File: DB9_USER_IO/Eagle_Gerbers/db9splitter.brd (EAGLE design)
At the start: 62.5 x 19.8 mm, 19 parts, among them IC1 74LVC1G04DBV

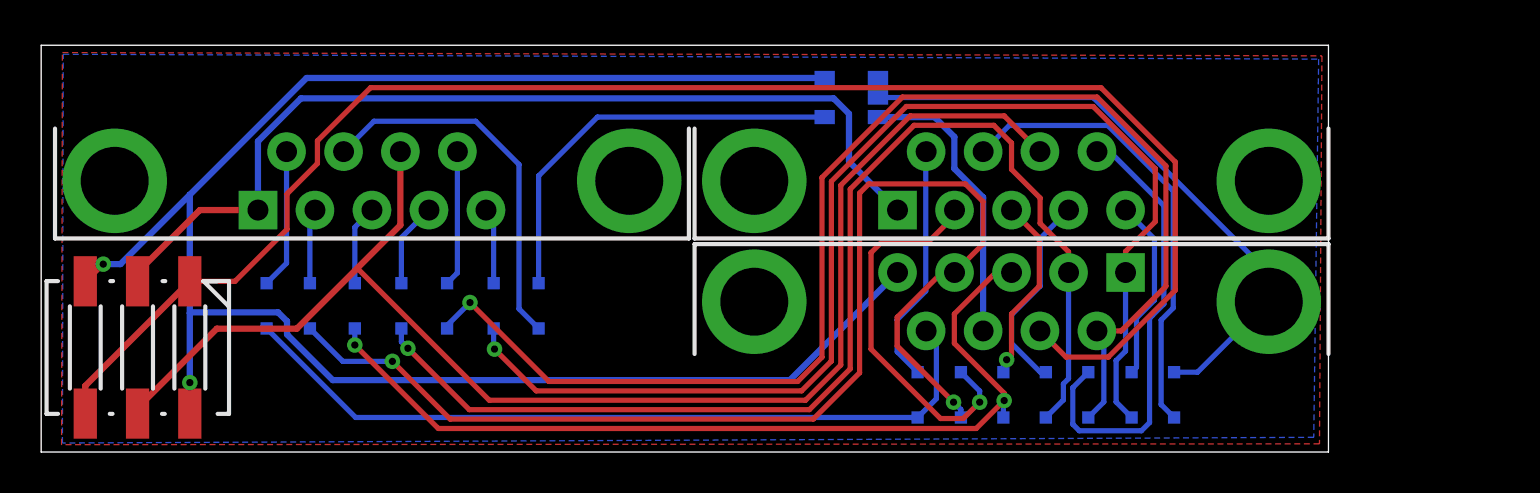
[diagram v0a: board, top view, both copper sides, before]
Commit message: updated db9splitter
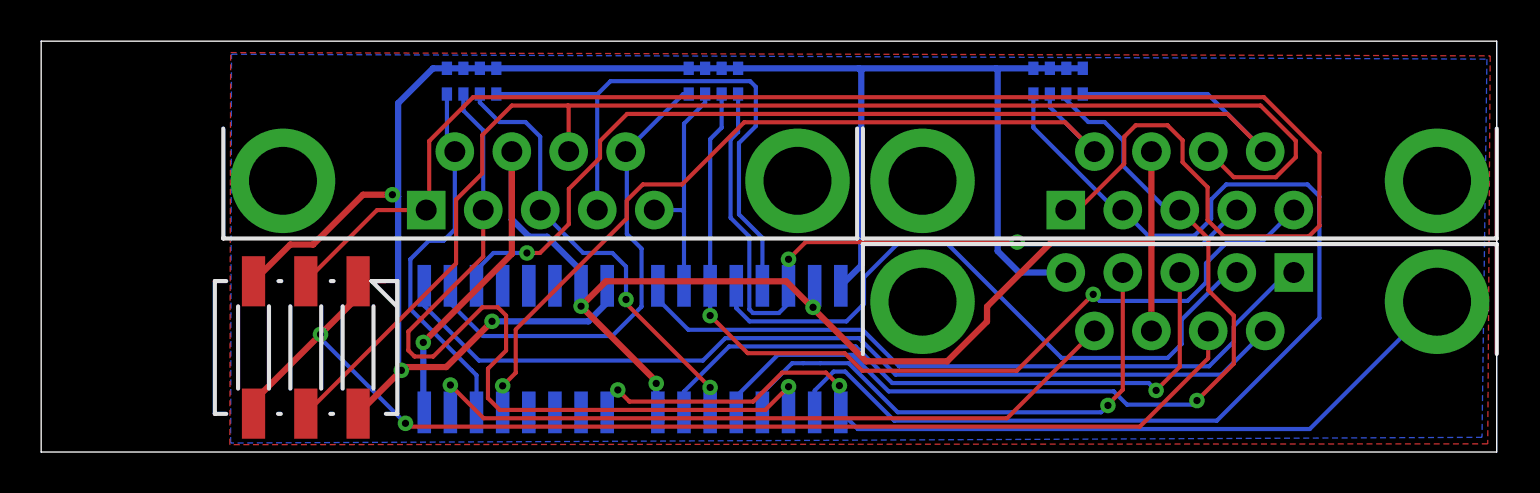
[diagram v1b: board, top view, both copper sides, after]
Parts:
- removed D1, D10, D11, D12, D13, D14, D2, D3, D4, D5, D6, D7, D8, D9: (no value), diode:SOD323-R
- removed IC1: 74LVC1G04DBV, 74xx-little-de:SOT23-5
- added IC2, IC3: 74HC157D, 74xx-eu:SO16
- added RN2, RN3, RN5: 10K, resistor-dil:0603-ARC
- moved J1 8.18 mm to (55.3, 13.2)
- moved J2 8.18 mm to (55.3, 7.30)
- moved J3 8.18 mm to (24.2, 13.2)
- moved S1 8.18 mm to (12.9, 5.08)
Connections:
- removed net /SELECT: D10.C, IC1.4
- removed net N$1: D13.C, J1.1
- removed net N$11: D6.C, J1.9
- removed net N$12: D5.C, J1.6
- removed net N$13: D12.C, J3.9
- removed net N$14: D11.C, J3.6
- removed net N$15: D4.A, J1.8
- removed net N$2: D14.C, J3.1
- removed net N$3: D2.C, J1.3
- removed net N$4: D8.C, J3.3
- removed net N$5: D1.C, J1.2
- removed net N$6: D3.C, J1.4
- removed net N$7: D7.C, J3.2
- removed net N$8: D9.C, J3.4
- removed net N$9: D10.A, J3.8
- new net 1PDOWN: IC2.14, J1.2, RN2.1
- new net 1PFIRE1: IC3.11, J1.6, RN5.1
- new net 1PFIRE2: IC3.5, J1.9, RN5.3
- new net 1PLEFT: IC2.5, J1.3, RN5.2
- new net 1PRIGHT: IC2.2, J1.4, RN5.4
- new net 1PUP: IC2.11, J1.1, RN2.2
- new net 2PDOWN: IC2.13, J3.2, RN3.1
- new net 2PFIRE1: IC3.10, J3.6, RN2.4
- new net 2PFIRE2: IC3.6, J3.9, RN3.4
- new net 2PLEFT: IC2.6, J3.3, RN3.2
- new net 2PRIGHT: IC2.3, J3.4, RN3.3
- new net 2PUP: IC2.10, J3.1, RN2.3
- net DOWN: now also IC2.12; no longer D1.A, D7.A
- net FIRE1: now also IC3.9; no longer D11.A, D5.A
- net FIRE2: now also IC3.7; no longer D12.A, D6.A
- net GND: now also IC2.15, IC2.8, IC3.15, IC3.8, J1.8, J3.8; no longer IC1.3
- net LEFT: now also IC2.7; no longer D2.A, D8.A
- net RIGHT: now also IC2.4; no longer D3.A, D9.A
- net SELECT: now also IC2.1, IC3.1; no longer D4.C, IC1.2
- net UP: now also IC2.9; no longer D13.A, D14.A
- net VCC: now also IC2.16, IC3.16, RN2.5, RN2.6, RN2.7, RN2.8, RN3.5, RN3.6, RN3.7, RN3.8, RN5.5, RN5.6, RN5.7, RN5.8; no longer IC1.5
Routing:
- net GND: track 14.1 -> 73.1 mm, vias 0 -> 4
- net 1PFIRE1: track 0.00 -> 54.5 mm, vias 0 -> 1
- net 1PRIGHT: track 0.00 -> 54.5 mm
- net 1PLEFT: track 0.00 -> 44.9 mm, vias 0 -> 1
- net 1PUP: track 0.00 -> 44.5 mm, vias 0 -> 2
- net 1PFIRE2: track 0.00 -> 41.4 mm, vias 0 -> 1
- net 2PRIGHT: track 0.00 -> 41.3 mm, vias 0 -> 1
- net 1PDOWN: track 0.00 -> 38.2 mm, vias 0 -> 2
- net RIGHT: track 58.6 -> 26.2 mm, vias 2 -> 1
- net PIN5: track 46.4 -> 78.3 mm
- net 2PDOWN: track 0.00 -> 30.0 mm
- net DOWN: track 57.8 -> 33.4 mm, vias 1 -> 0
- net UP: track 59.3 -> 35.3 mm, vias 1 -> 0
- net 2PFIRE1: track 0.00 -> 23.7 mm
- net N$15: track 22.6 -> 0.00 mm
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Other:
- board size 62.5 x 19.8 mm -> 70.7 x 20 mm
